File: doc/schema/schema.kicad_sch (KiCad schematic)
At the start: 18 parts, among them M1 Motor_DC, M2 Motor_DC, SW1 SW_Push, U1 L293D

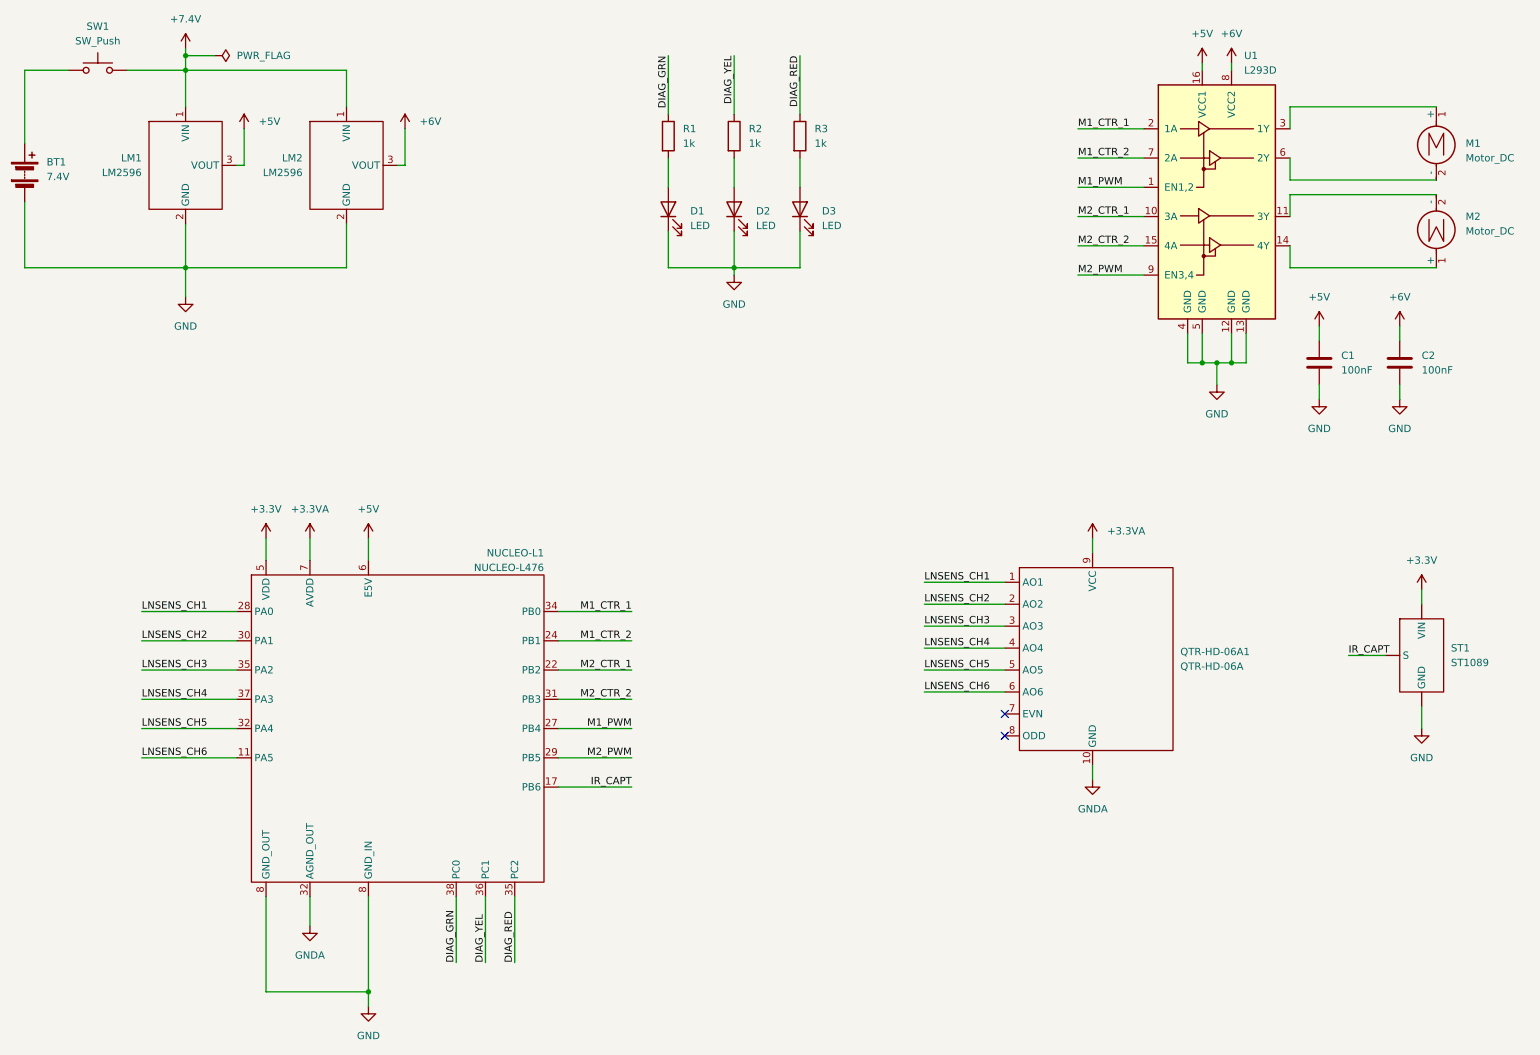
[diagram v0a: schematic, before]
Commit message: Documentation update
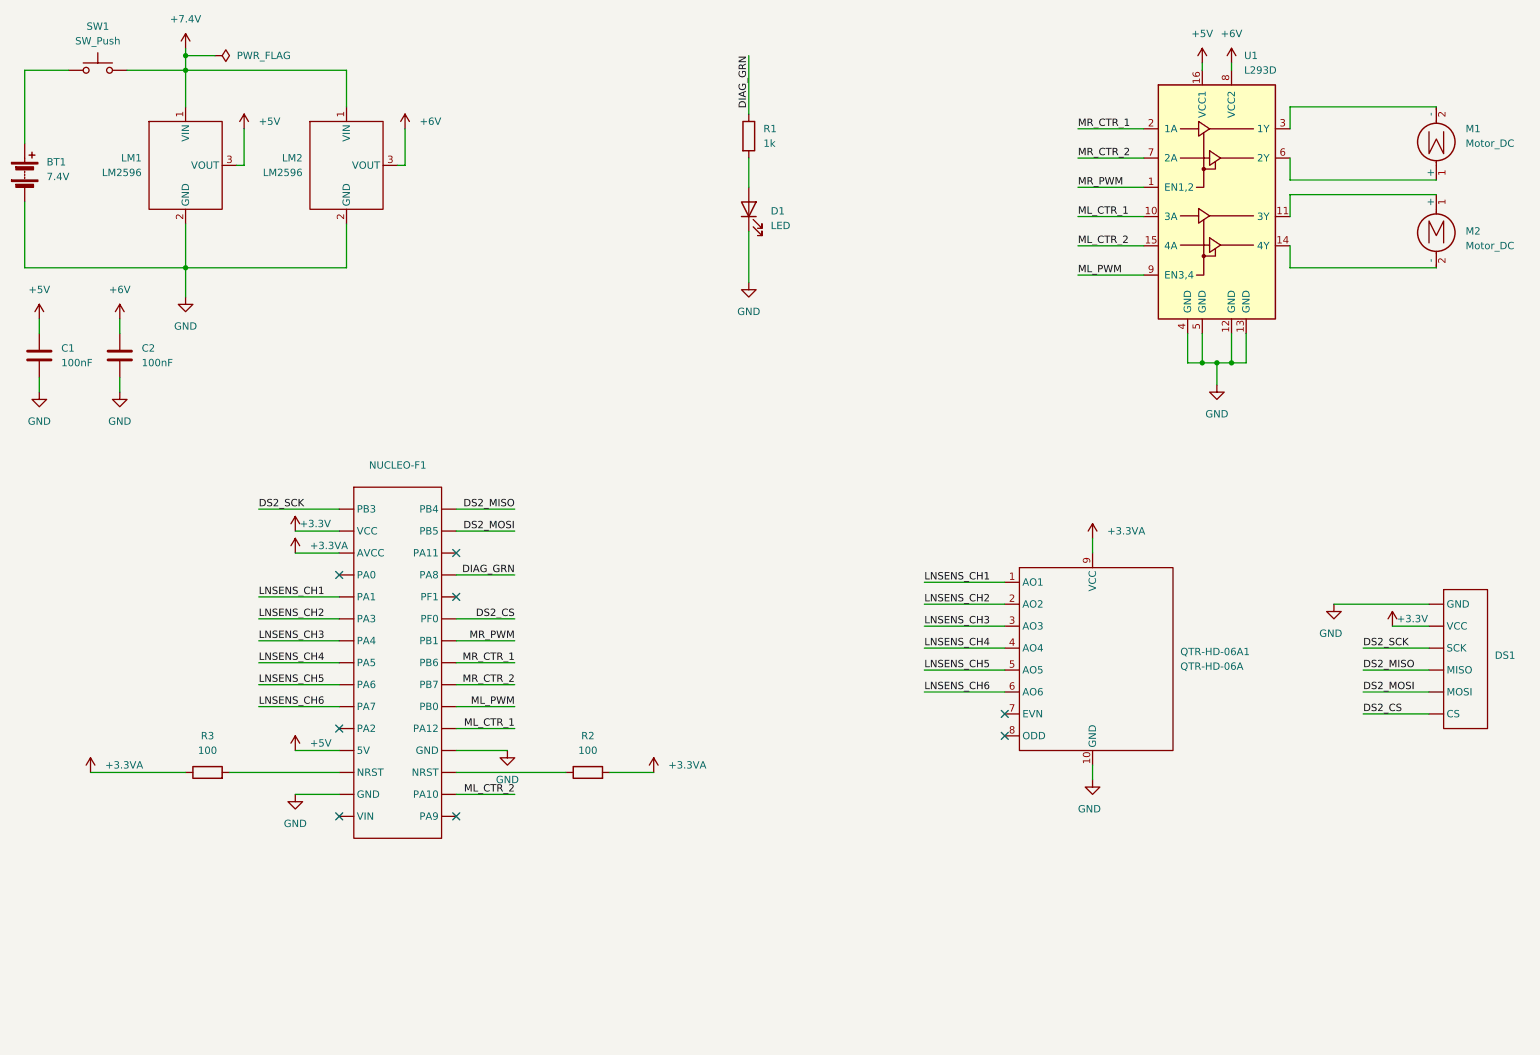
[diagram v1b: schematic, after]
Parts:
- removed D2, D3: LED, symbol Device:LED
- removed NUCLEO-L1: NUCLEO-L476, symbol route-runner:nucleo-l476
- removed ST1: ST1089, symbol route-runner:ST1089
- added DS1: ~, symbol route-runner:ds2-socket
- added NUCLEO-F1: ~, symbol route-runner:nucleo-f303
- R2, R3: value 1k -> 100
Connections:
- net DIAG_RED is gone; now on net +3.3VA: R3.1
- net GNDA is gone; now on net GND: QTR-HD-06A1.10 (GND)
- net +3.3V: now also DS1. (VCC), NUCLEO-F1. (VIN)
- net +3.3VA: now also R2.2, NUCLEO-F1. (VIN)
- net +5V: now also NUCLEO-F1. (VIN)
- net DIAG_GRN: now also NUCLEO-F1. (VIN)
- net GND: now also DS1. (VCC), NUCLEO-F1. (VIN)
- net LNSENS_CH1: now also NUCLEO-F1. (VIN)
- net LNSENS_CH2: now also NUCLEO-F1. (VIN)
- net LNSENS_CH3: now also NUCLEO-F1. (VIN)
- net LNSENS_CH4: now also NUCLEO-F1. (VIN)
- net LNSENS_CH5: now also NUCLEO-F1. (VIN)
- net LNSENS_CH6: now also NUCLEO-F1. (VIN)
- net at M2.1 (+): now also U1.11 (3Y); no longer U1.14 (4Y)
- net at M2.2 (-): now also U1.14 (4Y); no longer U1.11 (3Y)
- net at R3.2: now also NUCLEO-F1. (VIN)
- net at U1.3 (1Y): now also M1.2 (-); no longer M1.1 (+)
- net at U1.6 (2Y): now also M1.1 (+); no longer M1.2 (-)
- net DIAG_YEL: no longer names the net of R2.1
- net DIAG_YEL: now also NUCLEO-F1. (VIN)
- net M1_CTR_1 renamed MR_CTR_1
- net MR_CTR_1: now also NUCLEO-F1. (VIN)
- net M1_CTR_2 renamed MR_CTR_2
- net MR_CTR_2: now also NUCLEO-F1. (VIN)
- net M1_PWM renamed MR_PWM
- net MR_PWM: now also NUCLEO-F1. (VIN)
- net M2_CTR_1 renamed ML_CTR_1
- net ML_CTR_1: now also NUCLEO-F1. (VIN)
- net M2_CTR_2 renamed ML_CTR_2
- net ML_CTR_2: now also NUCLEO-F1. (VIN)
- net M2_PWM renamed ML_PWM
- net ML_PWM: now also NUCLEO-F1. (VIN)
- new net DS2_CS: DS1. (VCC), NUCLEO-F1. (VIN)
- new net DS2_MISO: DS1. (VCC), NUCLEO-F1. (VIN)
- new net DS2_MOSI: DS1. (VCC), NUCLEO-F1. (VIN)
- new net DS2_SCK: DS1. (VCC), NUCLEO-F1. (VIN)
- no-connect marks 2 -> 8
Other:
- moved on the sheet: C1, C2, D1, M1, M2, R1
